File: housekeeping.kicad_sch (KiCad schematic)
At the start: 9 parts, among them U15 LMR43620MSC5RPERQ1

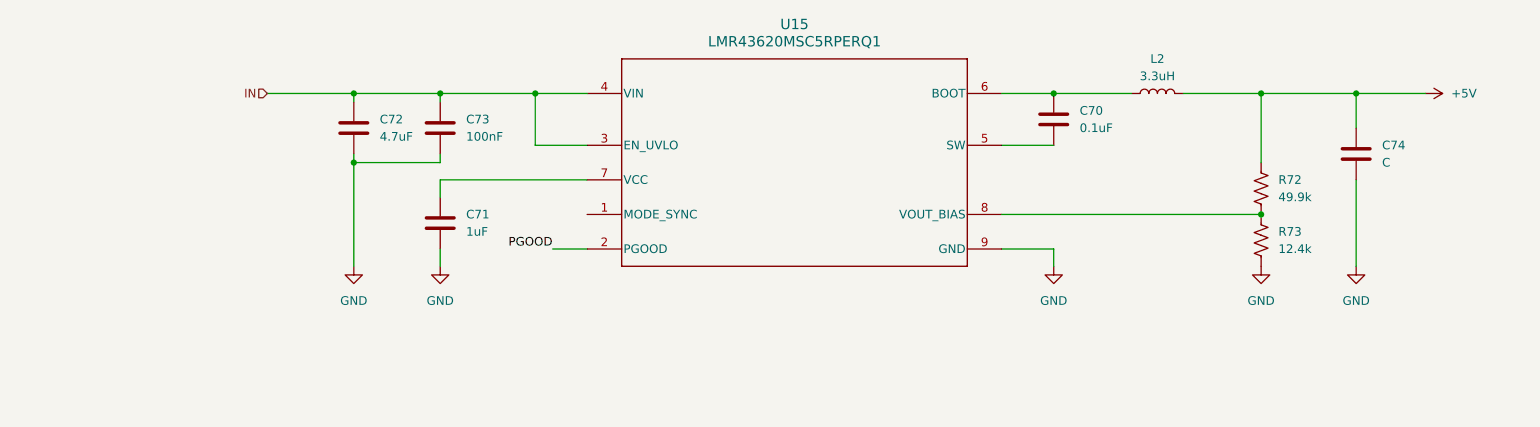
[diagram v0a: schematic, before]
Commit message: Adding control stuff
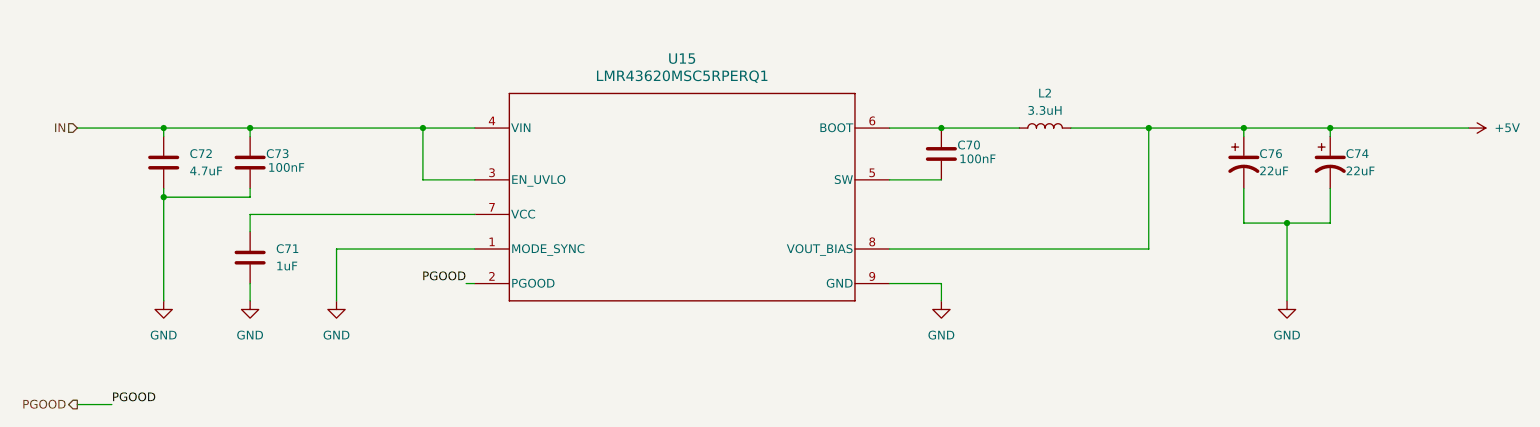
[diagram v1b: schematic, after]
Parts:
- removed C74: C, symbol Device:C
- removed R72: 49.9k, symbol Device:R_US
- removed R73: 12.4k, symbol Device:R_US
- added C74, C76: 22uF, Capacitor_SMD:CP_Elec_6.3x5.9, symbol Device:C_Polarized_US
- C70: value 0.1uF -> 100nF; footprint (none) -> Capacitor_SMD:C_0603_1608Metric; Mfr (none) -> KYOCERA AVX; Mfr P/N (none) -> 06035C104K4T2A; Supplier_1 (none) -> Digikey; Supplier_1 P/N (none) -> 478-KAM15AR71H104KTTR-ND; Supplier_1 Price @ Qty (none) -> 1; Supplier_1 Unit Price (none) -> 0.10000
- C71: footprint (none) -> Capacitor_SMD:C_0805_2012Metric; Mfr (none) -> Murata Electronics; Mfr P/N (none) -> GCM21BR71H105KA03K; Supplier_1 (none) -> Digikey; Supplier_1 P/N (none) -> 490-13310-2-ND; Supplier_1 Price @ Qty (none) -> 1; Supplier_1 Unit Price (none) -> 0.22000
- C72: footprint (none) -> Capacitor_SMD:C_0805_2012Metric; Mfr (none) -> Murata Electronics; Mfr P/N (none) -> GRT21BR61H475KE13L; Supplier_1 (none) -> Digikey; Supplier_1 P/N (none) -> 490-12394-2-ND; Supplier_1 Price @ Qty (none) -> 1; Supplier_1 Unit Price (none) -> 0.24000
- C73: footprint (none) -> Capacitor_SMD:C_0603_1608Metric; Mfr (none) -> KYOCERA AVX; Mfr P/N (none) -> 06035C104K4T2A; Supplier_1 (none) -> Digikey; Supplier_1 P/N (none) -> 478-KAM15AR71H104KTTR-ND; Supplier_1 Price @ Qty (none) -> 1; Supplier_1 Unit Price (none) -> 0.10000
- L2: footprint (none) -> Inductor_SMD:L_Bourns_SRN6045TA; Mfr (none) -> Bourns Inc.; Mfr P/N (none) -> SRN6045TA-3R3Y; Supplier_1 (none) -> Digikey; Supplier_1 P/N (none) -> SRN6045TA-3R3YTR-ND; Supplier_1 Price @ Qty (none) -> 1; Supplier_1 Unit Price (none) -> 0.45000
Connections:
- net +5V: now also U15.8 (VOUT_BIAS), C74.1, C76.1
- net GND: now also U15.1 (MODE_SYNC), C74.2, C76.2
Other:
- moved on the sheet: C71, C72, L2, U15
